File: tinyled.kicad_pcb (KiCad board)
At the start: 2 copper layers, 48.8 x 20.6 mm, 44 parts, among them J1 Conn_01x01_Female, J4 Conn_01x01_Female

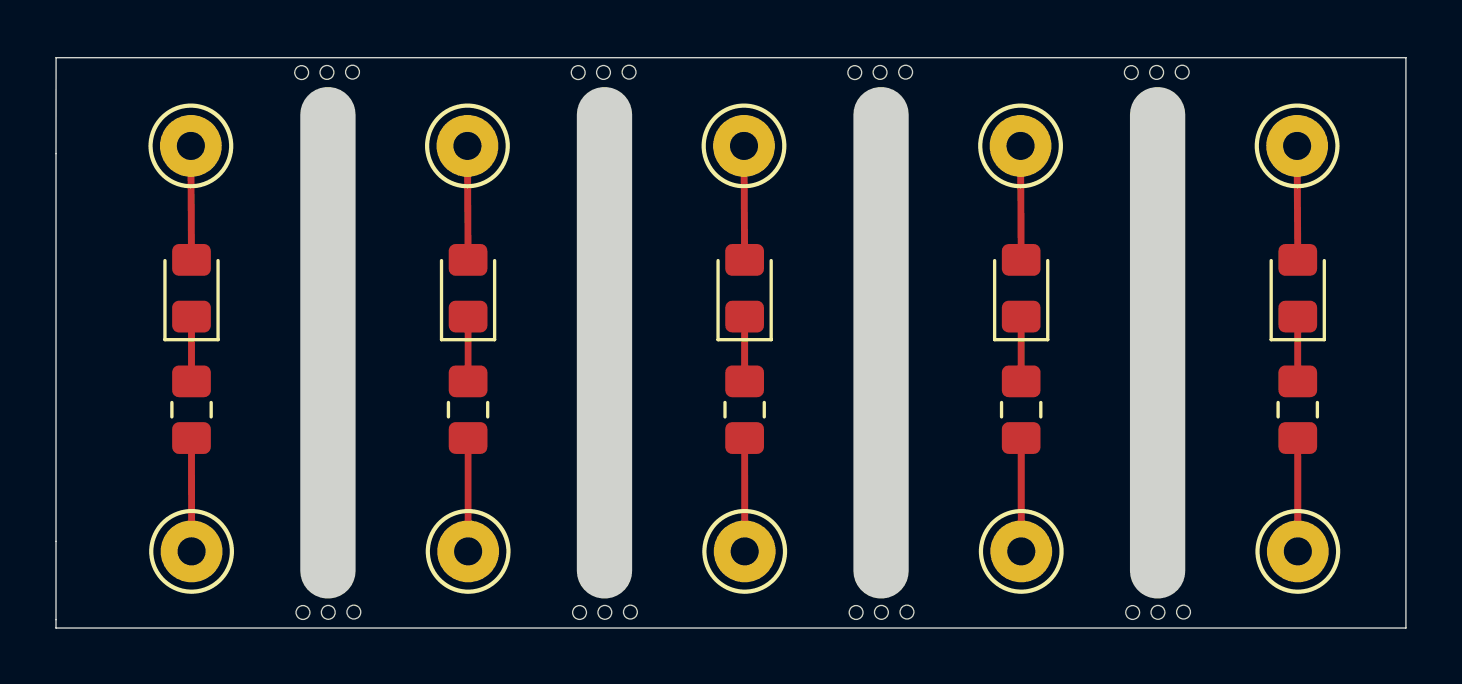
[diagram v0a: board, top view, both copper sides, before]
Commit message: rev2
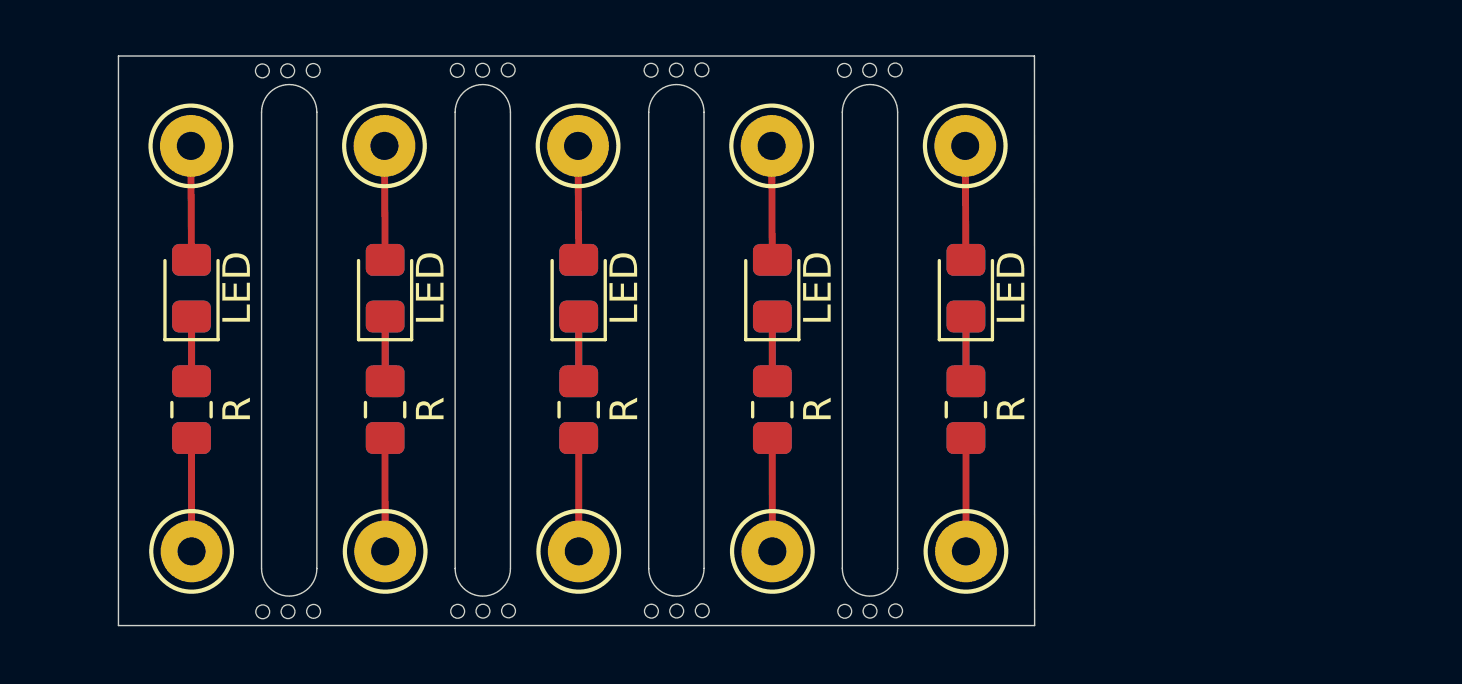
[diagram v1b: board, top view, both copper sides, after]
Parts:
- removed the D1 at (23.8, 84.0)
- removed the D1 at (13.8, 84.0)
- removed the D1 at (3.80, 84.0)
- removed the D1 at (-6.20, 84.0)
- removed the J1 at (23.8, 78.9)
- removed the J1 at (13.8, 78.9)
- removed the J1 at (3.78, 78.9)
- removed the J1 at (-6.22, 78.9)
- removed the J4 at (23.8, 93.5)
- removed the J4 at (13.8, 93.5)
- removed the J4 at (3.80, 93.5)
- removed the J4 at (-6.20, 93.5)
- removed the R1 at (23.8, 88.4)
- removed the R1 at (13.8, 88.4)
- removed the R1 at (3.80, 88.4)
- removed the R1 at (-6.20, 88.4)
- removed the V at (16.8, 75.0)
- removed the V at (18.7, 94.5)
- removed the V at (8.72, 94.5)
- removed the V at (-1.28, 94.5)
- removed the V at (17.7, 75.0)
- removed the V at (7.75, 75.0)
- removed the V at (-2.25, 75.0)
- removed the V at (17.8, 94.6)
- removed the V at (7.80, 94.6)
- removed the V at (-2.20, 94.6)
- removed the V at (-13.1, 94.6)
- removed the V at (6.84, 75.0)
- removed the V at (-11.3, 94.5)
- removed the V at (-12.2, 94.6)
- removed the V at (-3.16, 75.0)
- removed the V at (18.7, 75.0)
- removed the V at (8.67, 75.0)
- removed the V at (-1.33, 75.0)
- removed the V at (16.9, 94.6)
- removed the V at (6.88, 94.6)
- removed the V at (-3.12, 94.6)
- added D1: LED, Diode_SMD:D_0805_2012Metric_Pad1.15x1.40mm_HandSolder, B.Cu at (-16.2, 84.0)
- added D1: LED, Diode_SMD:D_0805_2012Metric_Pad1.15x1.40mm_HandSolder, F.Cu at (11.8, 84.0)
- added D1: LED, Diode_SMD:D_0805_2012Metric_Pad1.15x1.40mm_HandSolder, B.Cu at (-2.19, 84.0)
- added D1: LED, Diode_SMD:D_0805_2012Metric_Pad1.15x1.40mm_HandSolder, B.Cu at (-9.19, 84.0)
- added D1: LED, Diode_SMD:D_0805_2012Metric_Pad1.15x1.40mm_HandSolder, B.Cu at (4.81, 84.0)
- added D1: LED, Diode_SMD:D_0805_2012Metric_Pad1.15x1.40mm_HandSolder, B.Cu at (11.8, 84.0)
- added D1: LED, Diode_SMD:D_0805_2012Metric_Pad1.15x1.40mm_HandSolder, F.Cu at (-9.20, 84.0)
- added D1: LED, Diode_SMD:D_0805_2012Metric_Pad1.15x1.40mm_HandSolder, F.Cu at (-2.20, 84.0)
- added D1: LED, Diode_SMD:D_0805_2012Metric_Pad1.15x1.40mm_HandSolder, F.Cu at (4.80, 84.0)
- added J1: Conn_01x01_Female, Wickerlib:CONN-HEADER-STRAIGHT-P2.54MM-1x01, F.Cu at (-9.22, 78.9)
- added J1: Conn_01x01_Female, Wickerlib:CONN-HEADER-STRAIGHT-P2.54MM-1x01, F.Cu at (-2.22, 78.9)
- added J1: Conn_01x01_Female, Wickerlib:CONN-HEADER-STRAIGHT-P2.54MM-1x01, F.Cu at (4.78, 78.9)
- added J1: Conn_01x01_Female, Wickerlib:CONN-HEADER-STRAIGHT-P2.54MM-1x01, F.Cu at (11.8, 78.9)
- added J4: Conn_01x01_Female, Wickerlib:CONN-HEADER-STRAIGHT-P2.54MM-1x01, F.Cu at (-9.20, 93.5)
- added J4: Conn_01x01_Female, Wickerlib:CONN-HEADER-STRAIGHT-P2.54MM-1x01, F.Cu at (-2.20, 93.5)
- added J4: Conn_01x01_Female, Wickerlib:CONN-HEADER-STRAIGHT-P2.54MM-1x01, F.Cu at (4.80, 93.5)
- added J4: Conn_01x01_Female, Wickerlib:CONN-HEADER-STRAIGHT-P2.54MM-1x01, F.Cu at (11.8, 93.5)
- added R1: R, Resistor_SMD:R_0805_2012Metric_Pad1.15x1.40mm_HandSolder, B.Cu at (-2.19, 88.4)
- added R1: R, Resistor_SMD:R_0805_2012Metric_Pad1.15x1.40mm_HandSolder, F.Cu at (11.8, 88.4)
- added R1: R, Resistor_SMD:R_0805_2012Metric_Pad1.15x1.40mm_HandSolder, B.Cu at (-16.2, 88.4)
- added R1: R, Resistor_SMD:R_0805_2012Metric_Pad1.15x1.40mm_HandSolder, B.Cu at (-9.19, 88.4)
- added R1: R, Resistor_SMD:R_0805_2012Metric_Pad1.15x1.40mm_HandSolder, B.Cu at (4.81, 88.4)
- added R1: R, Resistor_SMD:R_0805_2012Metric_Pad1.15x1.40mm_HandSolder, B.Cu at (11.8, 88.4)
- added R1: R, Resistor_SMD:R_0805_2012Metric_Pad1.15x1.40mm_HandSolder, F.Cu at (-9.20, 88.4)
- added R1: R, Resistor_SMD:R_0805_2012Metric_Pad1.15x1.40mm_HandSolder, F.Cu at (-2.20, 88.4)
- added R1: R, Resistor_SMD:R_0805_2012Metric_Pad1.15x1.40mm_HandSolder, F.Cu at (4.80, 88.4)
- added V: HOLE-PLATED-200MIL, Wickerlib:HOLE-UNPLATED-200MIL, F.Cu at (-0.52, 94.5)
- added V: HOLE-PLATED-200MIL, Wickerlib:HOLE-UNPLATED-200MIL, F.Cu at (-13.7, 94.5)
- added V: HOLE-PLATED-200MIL, Wickerlib:HOLE-UNPLATED-200MIL, F.Cu at (-6.61, 94.5)
- added V: HOLE-PLATED-200MIL, Wickerlib:HOLE-UNPLATED-200MIL, F.Cu at (1.32, 94.5)
- added V: HOLE-PLATED-200MIL, Wickerlib:HOLE-UNPLATED-200MIL, F.Cu at (6.46, 75.0)
- added V: HOLE-PLATED-200MIL, Wickerlib:HOLE-UNPLATED-200MIL, F.Cu at (7.37, 75.0)
- added V: HOLE-PLATED-200MIL, Wickerlib:HOLE-UNPLATED-200MIL, F.Cu at (8.30, 74.9)
- added V: HOLE-PLATED-200MIL, Wickerlib:HOLE-UNPLATED-200MIL, F.Cu at (1.31, 74.9)
- added V: HOLE-PLATED-200MIL, Wickerlib:HOLE-UNPLATED-200MIL, F.Cu at (-0.53, 75.0)
- added V: HOLE-PLATED-200MIL, Wickerlib:HOLE-UNPLATED-200MIL, F.Cu at (0.38, 74.9)
- added V: HOLE-PLATED-200MIL, Wickerlib:HOLE-UNPLATED-200MIL, F.Cu at (-5.70, 74.9)
- added V: HOLE-PLATED-200MIL, Wickerlib:HOLE-UNPLATED-200MIL, F.Cu at (-5.68, 94.5)
- added V: HOLE-PLATED-200MIL, Wickerlib:HOLE-UNPLATED-200MIL, F.Cu at (-7.54, 75.0)
- added V: HOLE-PLATED-200MIL, Wickerlib:HOLE-UNPLATED-200MIL, F.Cu at (-6.62, 75.0)
- added V: HOLE-PLATED-200MIL, Wickerlib:HOLE-UNPLATED-200MIL, F.Cu at (-7.52, 94.5)
- added V: HOLE-PLATED-200MIL, Wickerlib:HOLE-UNPLATED-200MIL, F.Cu at (6.47, 94.5)
- added V: HOLE-PLATED-200MIL, Wickerlib:HOLE-UNPLATED-200MIL, F.Cu at (7.39, 94.5)
- added V: HOLE-PLATED-200MIL, Wickerlib:HOLE-UNPLATED-200MIL, F.Cu at (-12.7, 94.5)
- added V: HOLE-PLATED-200MIL, Wickerlib:HOLE-UNPLATED-200MIL, F.Cu at (0.40, 94.5)
- added V: HOLE-PLATED-200MIL, Wickerlib:HOLE-UNPLATED-200MIL, F.Cu at (8.31, 94.5)
- added V: HOLE-PLATED-200MIL, Wickerlib:HOLE-UNPLATED-200MIL, F.Cu at (-14.6, 94.5)
- moved V 1.42 mm to (-12.7, 75.0)
- moved V 1.42 mm to (-14.6, 75.0)
- moved V 1.42 mm to (-13.7, 75.0)
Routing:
- net Net-(D1-Pad1): track 11.7 -> 23.4 mm
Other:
- board size 48.8 x 20.6 mm -> 33.1 x 20.6 mm
